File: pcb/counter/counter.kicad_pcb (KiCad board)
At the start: 2 copper layers, 91.4 x 51.8 mm, 17 parts, among them J1 Conn_01x01, J2 Conn_01x01, J3 Conn_01x01, J4 Conn_01x06, J5 Conn_01x02, J6 Conn_01x05, J7 Conn_01x03, Q1 Q_NPN_CBE, U1 74HC08

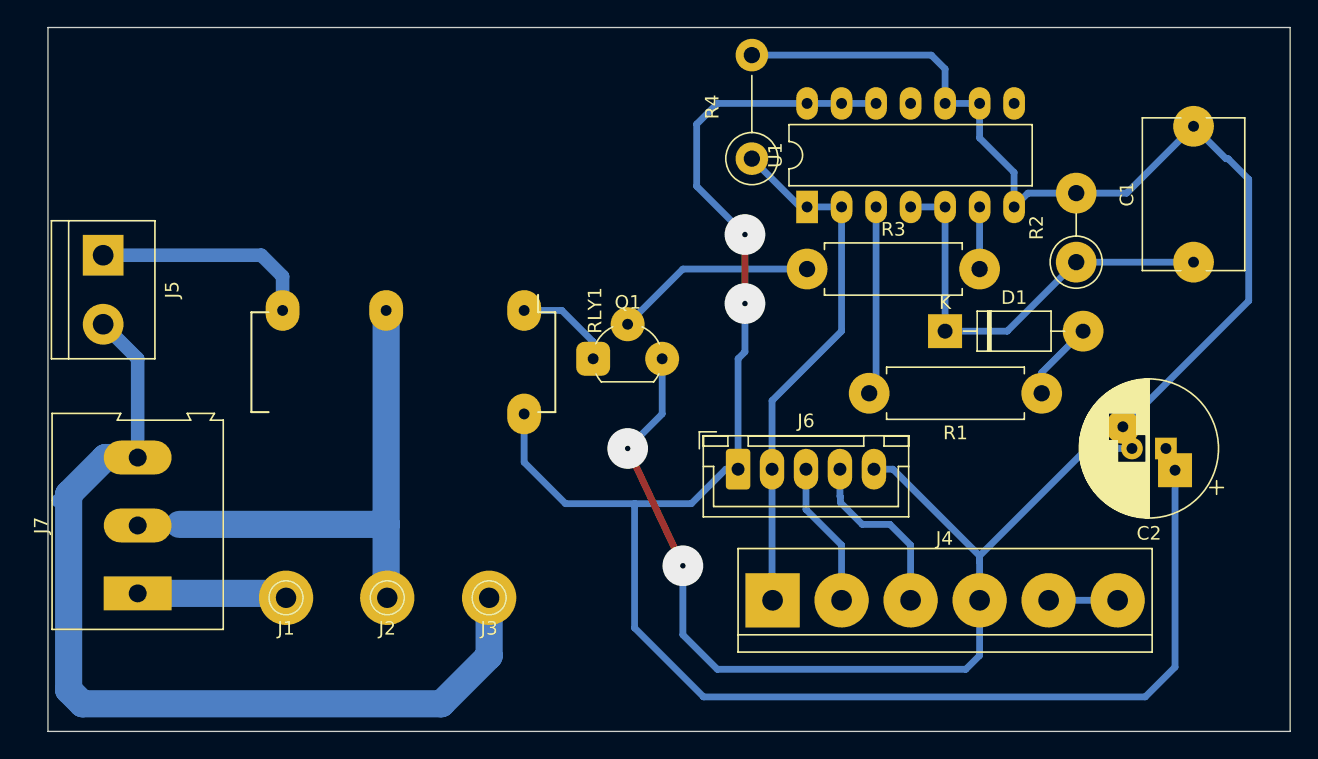
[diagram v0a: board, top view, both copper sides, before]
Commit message: Update.
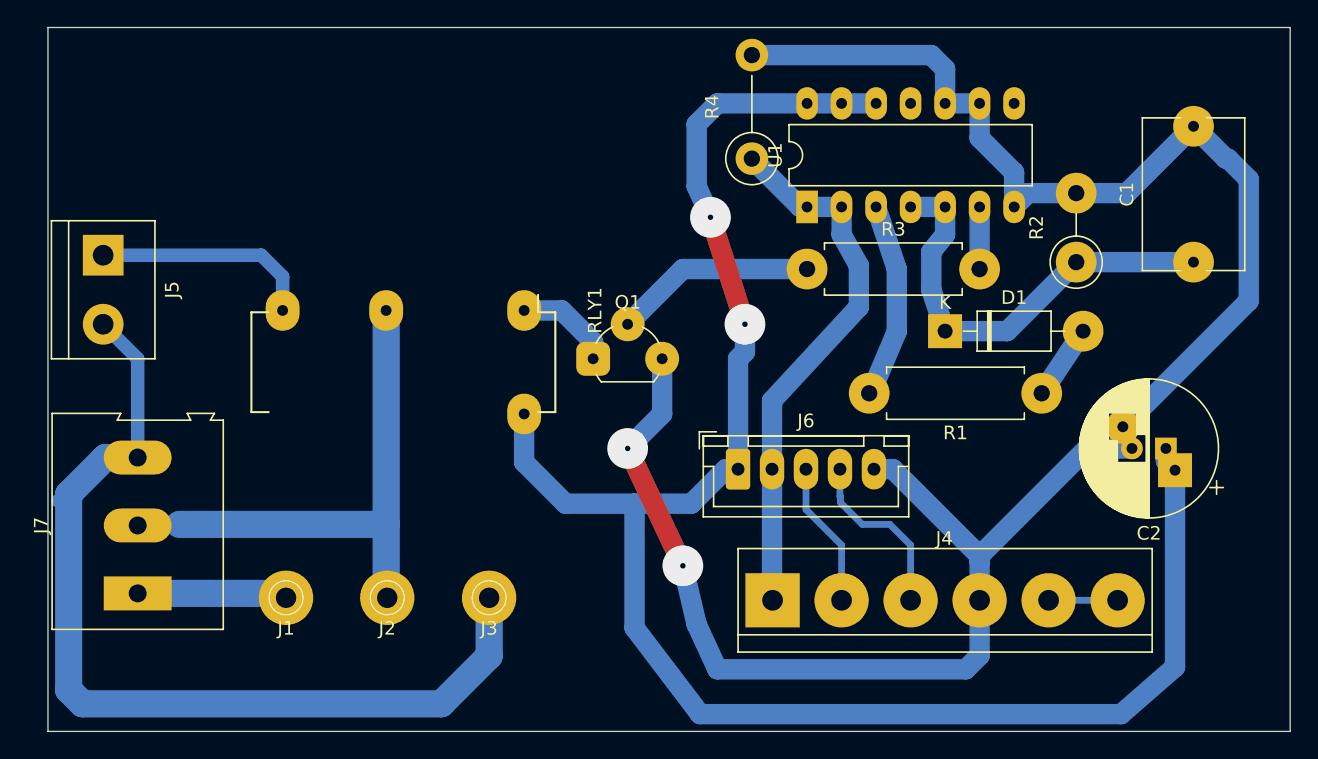
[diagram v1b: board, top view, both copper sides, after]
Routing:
- net Net-(R1-Pad2): track 13.9 -> 14.9 mm
- net Net-(J4-Pad1): track 39.2 -> 39.9 mm
- net GND: track 151.5 -> 150.9 mm
- net +5V: track 130.9 -> 131.4 mm
- net Net-(C1-Pad1): track 32.1 -> 32.6 mm
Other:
- net class Default removed
